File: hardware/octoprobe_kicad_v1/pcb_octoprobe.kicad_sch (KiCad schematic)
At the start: 12 parts, among them J101 Conn_01x20, J102 Conn_01x20, J103 Conn_01x20, J104 Conn_01x20, J105 Conn_01x20

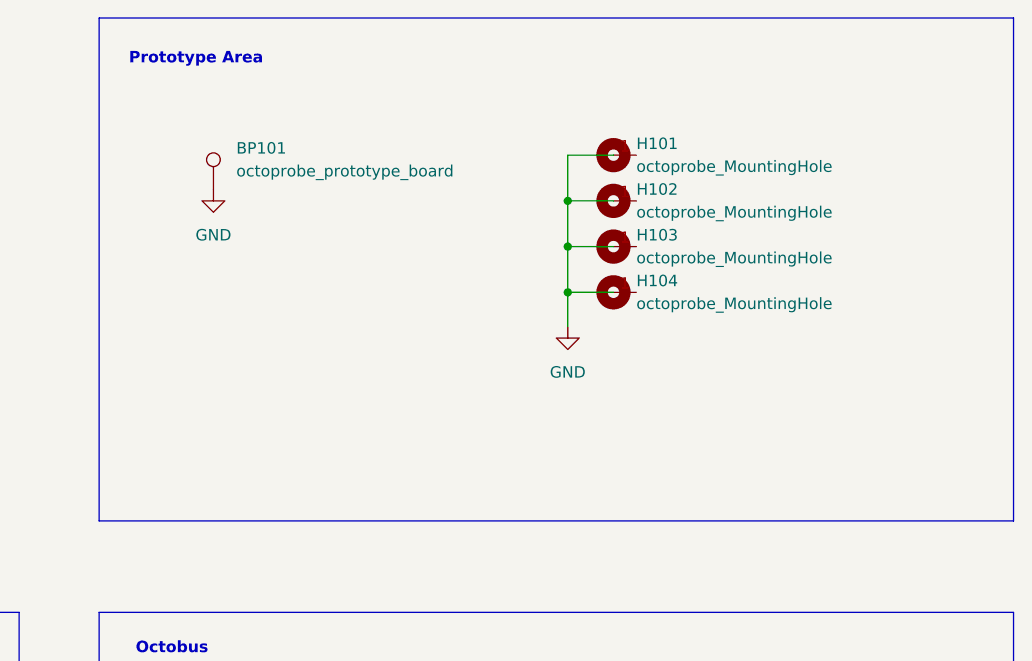
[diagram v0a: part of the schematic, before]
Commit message: Cable Tie
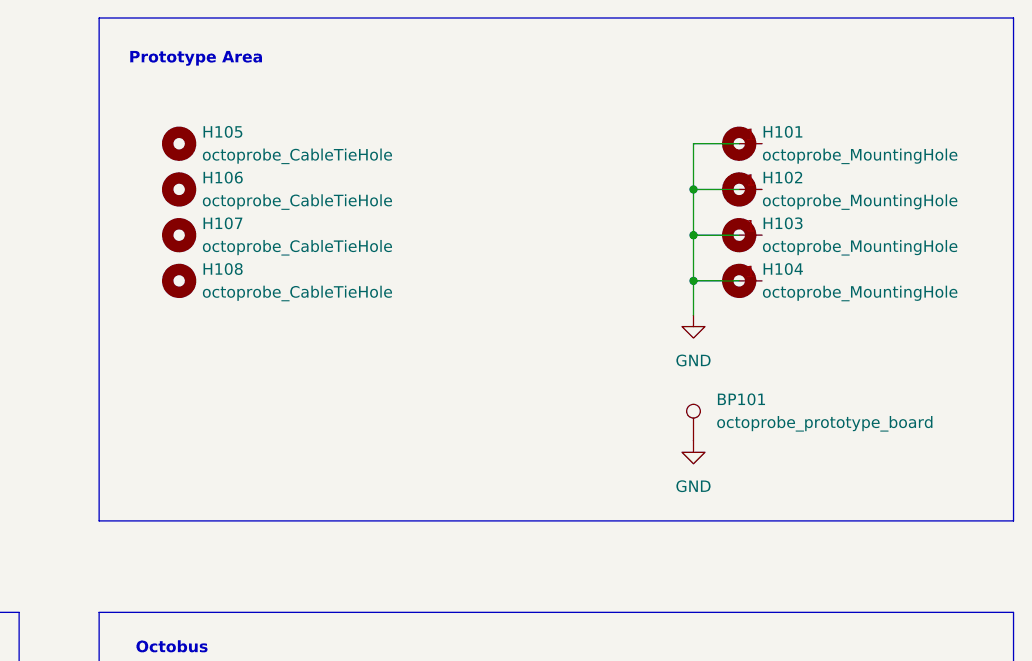
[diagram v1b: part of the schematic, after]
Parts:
- added H105, H106, H107, H108: octoprobe_CableTieHole, 00_project_library:octoprobe_CableTieHole, symbol 00_project_library:octoprobe_CableTieHole
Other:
- moved on the sheet: BP101, H101, H102, H103, H104

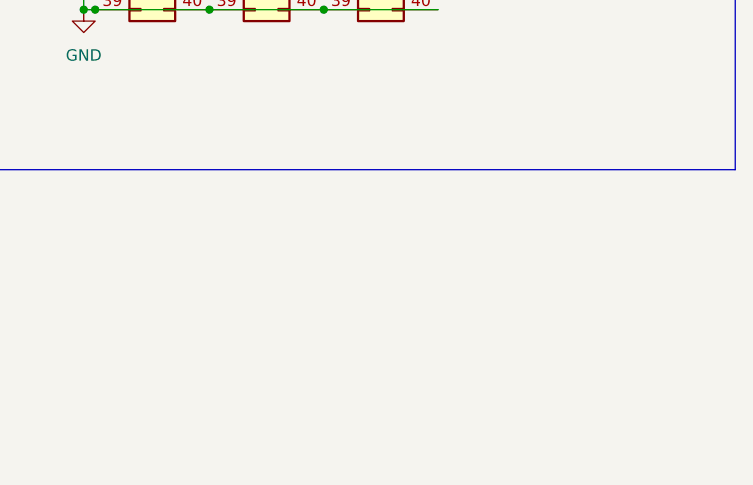
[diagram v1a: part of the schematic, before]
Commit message: PCB octoprobe tentacle v1.0
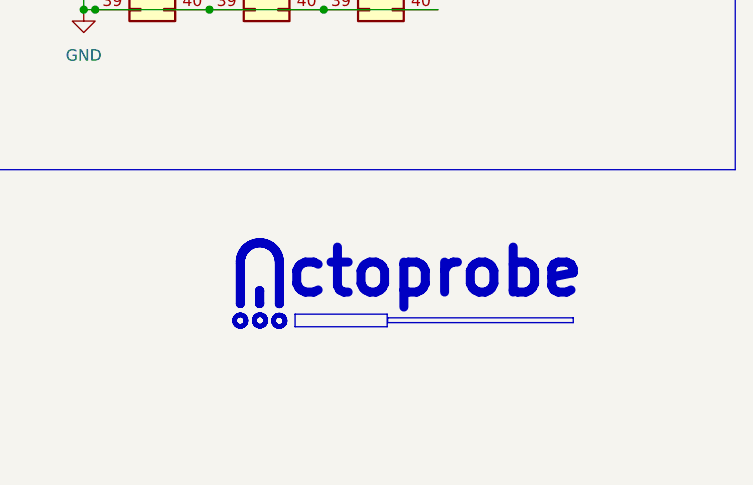
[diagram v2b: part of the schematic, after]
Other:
- title: Octoprobe -> Octoprobe tentacle
